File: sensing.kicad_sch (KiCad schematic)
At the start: 0 parts

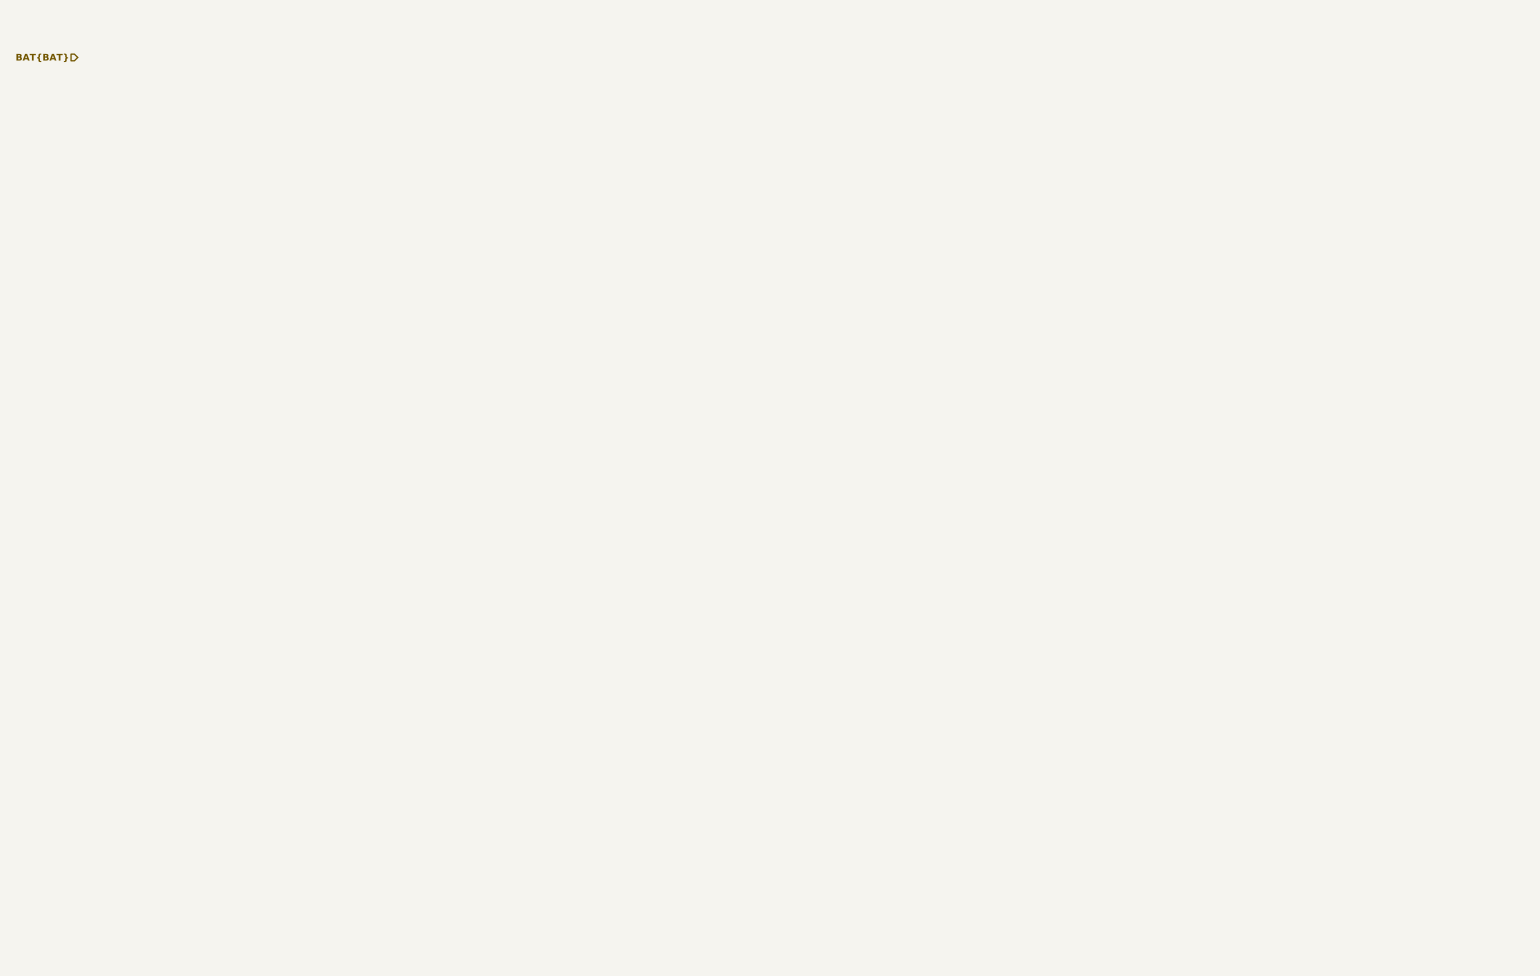
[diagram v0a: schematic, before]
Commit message: stuff
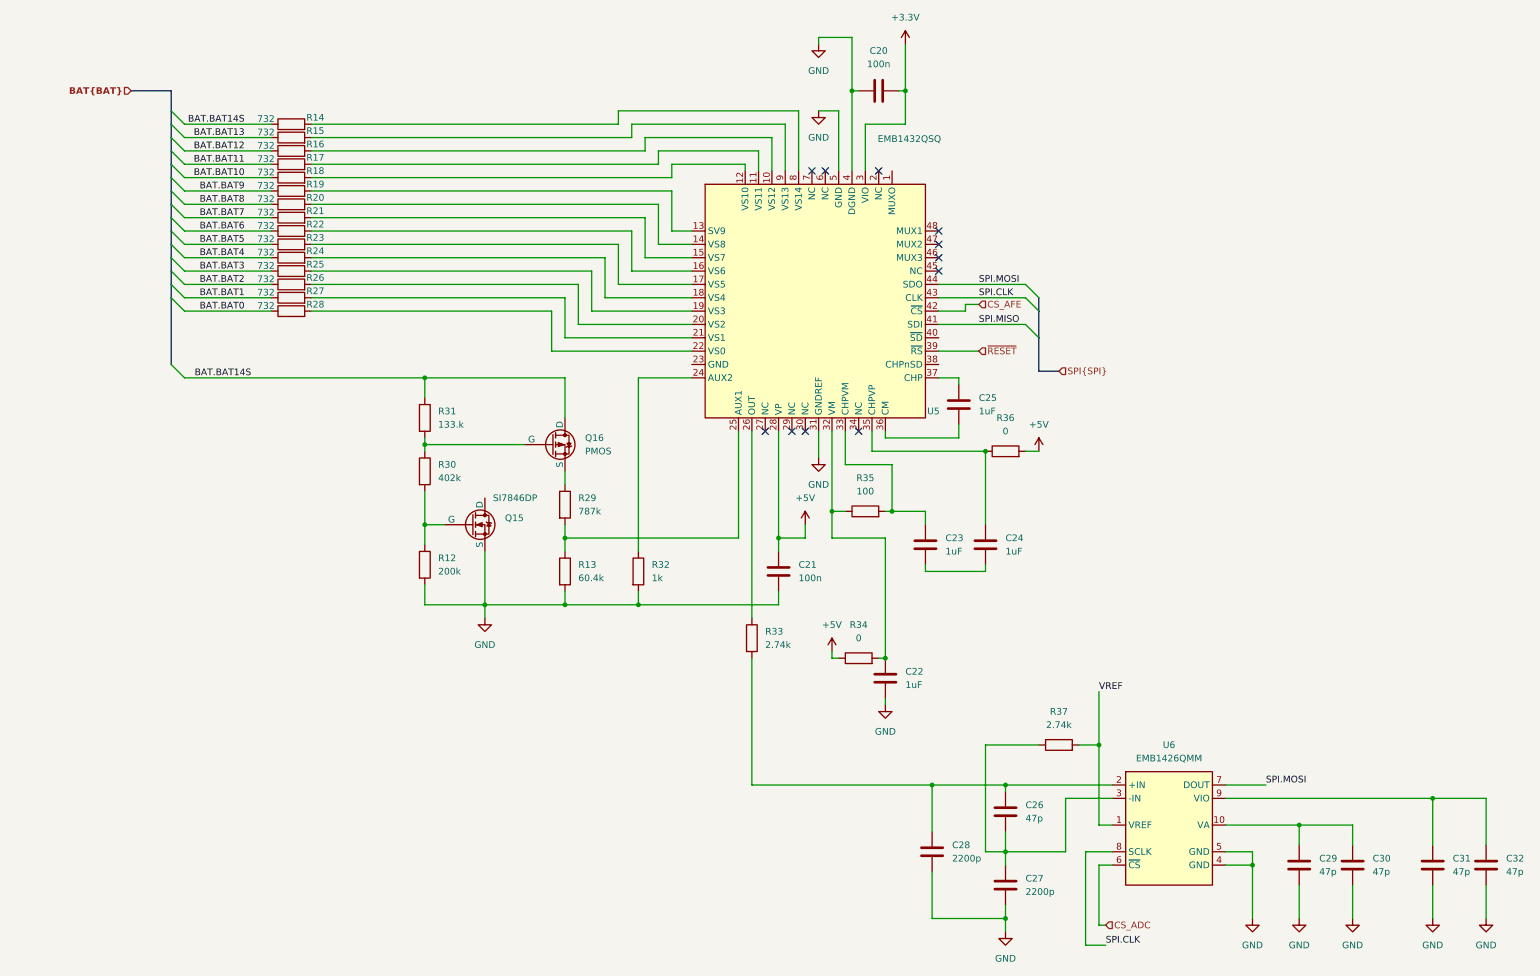
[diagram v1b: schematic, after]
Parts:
- added C20, C21: 100n, symbol Device:C
- added C22, C23, C24, C25: 1uF, symbol Device:C
- added C26, C29, C30, C31, C32: 47p, symbol Device:C
- added C27, C28: 2200p, symbol Device:C
- added Q15: SI7846DP, symbol Simulation_SPICE:NMOS
- added Q16: PMOS, symbol Simulation_SPICE:PMOS
- added R12: 200k, symbol Device:R
- added R13: 60.4k, symbol Device:R
- added R14, R15, R16, R17, R18, R19, R20, R21, R22, R23, R24, R25, R26, R27, R28: 732, symbol Device:R
- added R29: 787k, symbol Device:R
- added R30: 402k, symbol Device:R
- added R31: 133.k, symbol Device:R
- added R32: 1k, symbol Device:R
- added R33, R37: 2.74k, symbol Device:R
- added R34, R36: 0, symbol Device:R
- added R35: 100, symbol Device:R
- added U5: EMB1432QSQ, symbol samir:EMB1432QSQ
- added U6: EMB1426QMM, symbol samir:EMB1426QMM
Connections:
- new net: R27.2, U5.21 (VS1)
- new net: C26.2, C27.1, R37.1, U6.3 (-IN)
- new net: C31.1, C32.1, U6.9 (VIO)
- new net: R33.1, U5.26 (OUT)
- new net: C26.1, C28.1, R33.2, U6.2 (+IN)
- new net: R23.2, U5.17 (VS5)
- new net: R20.2, U5.14 (VS8)
- new net: R22.2, U5.16 (VS6)
- new net: R19.2, U5.13 (SV9)
- new net: Q16.2 (G), R30.1, R31.2
- new net: Q16.3 (S), R29.1
- new net: C24.1, R36.1, U5.35 (CHPVP)
- new net: C23.2, C24.2
- new net: C22.1, R34.2, R35.1, U5.32 (VM)
- new net: R24.2, U5.18 (VS4)
- new net: R26.2, U5.20 (VS2)
- new net: R25.2, U5.19 (VS3)
- new net: R32.1, U5.24 (AUX2)
- new net: C23.1, R35.2, U5.33 (CHPVM)
- new net: C29.1, C30.1, U6.10 (VA)
- new net: R17.2, U5.11 (VS11)
- new net: R15.2, U5.9 (VS13)
- new net: R28.2, U5.22 (VS0)
- new net: R21.2, U5.15 (VS7)
- new net: R16.2, U5.10 (VS12)
- new net: R18.2, U5.12 (VS10)
- new net: R13.1, R29.2, U5.25 (AUX1)
- new net: C25.2, U5.36 (CM)
- new net: C25.1, U5.37 (CHP)
- new net: R14.2, U5.8 (VS14)
- new net: Q15.2 (G), R12.1, R30.2
- new net +3.3V: C20.2, U5.3 (VIO)
- new net +5V: C21.1, R34.1, R36.2, U5.28 (VP)
- new net BAT.BAT0: R28.1
- new net BAT.BAT1: R27.1
- new net BAT.BAT10: R18.1
- new net BAT.BAT11: R17.1
- new net BAT.BAT12: R16.1
- new net BAT.BAT13: R15.1
- new net BAT.BAT14S: Q16.1 (D), R14.1, R31.1
- new net BAT.BAT2: R26.1
- new net BAT.BAT3: R25.1
- new net BAT.BAT4: R24.1
- new net BAT.BAT5: R23.1
- new net BAT.BAT6: R22.1
- new net BAT.BAT7: R21.1
- new net BAT.BAT8: R20.1
- new net BAT.BAT9: R19.1
- new net CS_ADC: U6.6 (~{CS})
- new net CS_AFE: U5.42 (~{CS})
- new net GND: C20.1, C21.2, C22.2, C27.2, C28.2, C29.2, C30.2, C31.2, C32.2, Q15.3 (S), R12.2, R13.2, R32.2, U5.31 (GNDREF), U5.4 (DGND), U5.5 (GND), U6.4 (GND), U6.5 (GND)
- new net SPI.CLK: U5.43 (CLK), U6.8 (SCLK)
- new net SPI.MISO: U5.41 (SDI)
- new net SPI.MOSI: U5.44 (SDO), U6.7 (DOUT)
- new net VREF: R37.2, U6.1 (VREF)
- new net ~{RESET}: U5.39 (~{RS})
- no-connect marks 0 -> 11
